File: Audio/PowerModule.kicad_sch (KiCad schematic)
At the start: 15 parts, among them J4 PWR_IN, J5 PWR_OUT

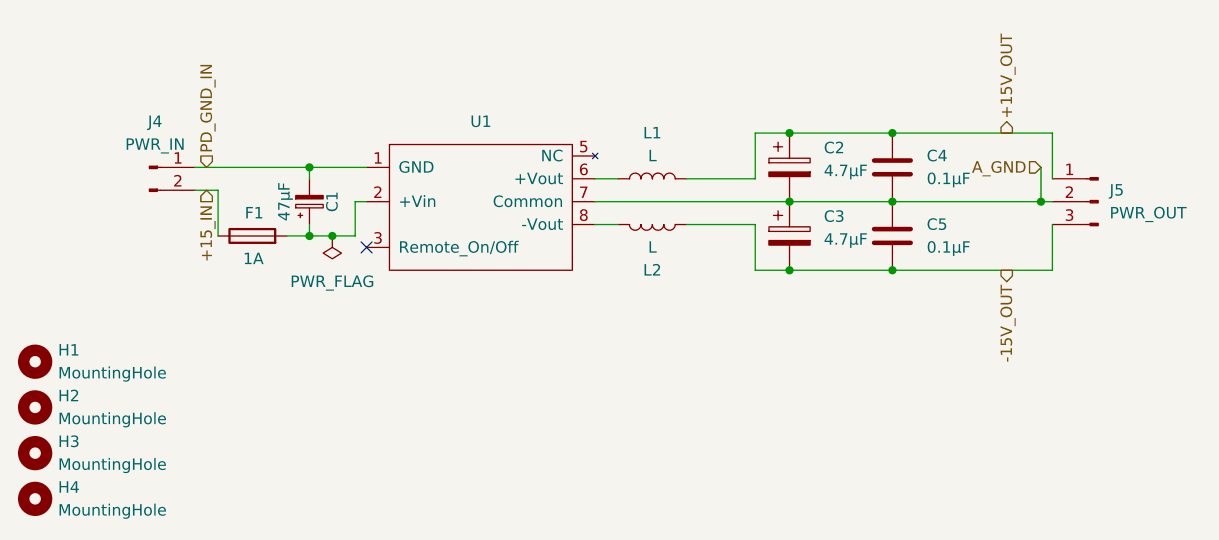
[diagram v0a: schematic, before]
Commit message: remove analyze
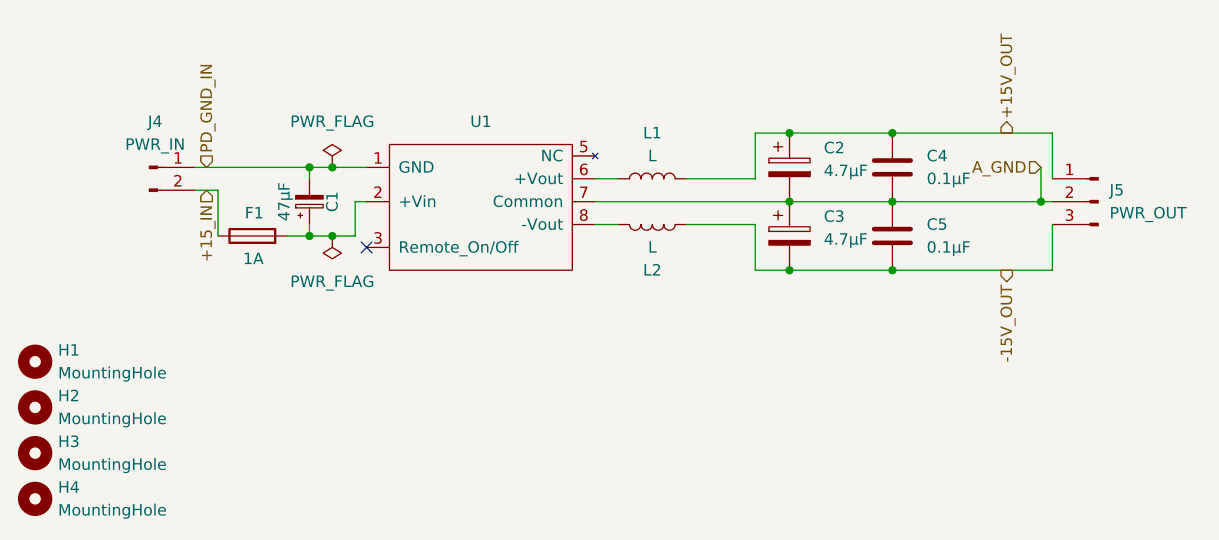
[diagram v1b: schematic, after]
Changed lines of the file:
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@@
+	)
+	(junction
+		(at 48.26 36.83)
+		(diameter 0)
+		(color 0 0 0 0)
 	)
 	(junction
@@
 	(wire
 		(pts
-			(xy 45.72 36.83) (xy 52.07 36.83)
+			(xy 45.72 36.83) (xy 48.26 36.83)
 		)
 		(stroke
@@
 		(pts
 			(xy 99.06 33.02) (xy 110.49 33.02)
+		)
+		(stroke
+			(width 0)
+			(type default)
+		)
+	)
+	(wire
+		(pts
+			(xy 48.26 36.83) (xy 52.07 36.83)
 		)
 		(stroke
@@
 					(unit 1)
 				)
+			)
+		)
+	)
+	(symbol
+		(lib_id "power:PWR_FLAG")
+		(at 48.26 36.83 0)
+		(unit 1)
+		(body_style 1)
+		(exclude_from_sim no)
+		(in_bom yes)
+		(on_board yes)
+		(in_pos_files yes)
+		(dnp no)
+		(fields_autoplaced yes)
+		(property "Reference" "#FLG08"
+			(at 48.26 34.925 0)
+			(hide yes)
+			(show_name no)
+			(do_not_autoplace no)
+			(effects
+				(font
+					(size 1.27 1.27)
+				)
+			)
+		)
+		(property "Value" "PWR_FLAG"
+			(at 48.26 31.75 0)
+			(show_name no)
+			(do_not_autoplace no)
+			(effects
+				(font
+					(size 1.27 1.27)
+				)
+			)
+		)
+		(property "Footprint" ""
+			(at 48.26 36.83 0)
+			(hide yes)
+			(show_name no)
+			(do_not_autoplace no)
+			(effects
+				(font
+					(size 1.27 1.27)
+				)
+			)
+		)
+		(property "Datasheet" ""
+			(at 48.26 36.83 0)
+			(hide yes)
+			(show_name no)
+			(do_not_autoplace no)
+			(effects
+				(font
+					(size 1.27 1.27)
+				)
+			)
+		)
+		(property "Description" "Special symbol for telling ERC where power comes from"
+			(at 48.26 36.83 0)
+			(hide yes)
+			(show_name no)
+			(do_not_autoplace no)
+			(effects
+				(font
+					(size 1.27 1.27)
+				)
+			)
+		)
+		(pin "1"
+		)
+		(instances
+			(project "AudioCase"
+				(path "/760b9589-09e7-434e-9ca2-6e4136e3b7a2/c17b312b-fe0a-430c-8356-b220c9b28aff"
+					(reference "#FLG08")
+					(unit 1)
+				)
